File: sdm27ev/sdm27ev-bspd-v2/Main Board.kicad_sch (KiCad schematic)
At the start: 41 parts, among them IC201 74AHC1G08, IC202 SN74LVC1G17DBVRG4, IC203 SN74HC32PWR, IC204 L7805ACD2T-TR, U201 TLV9022QDRQ1

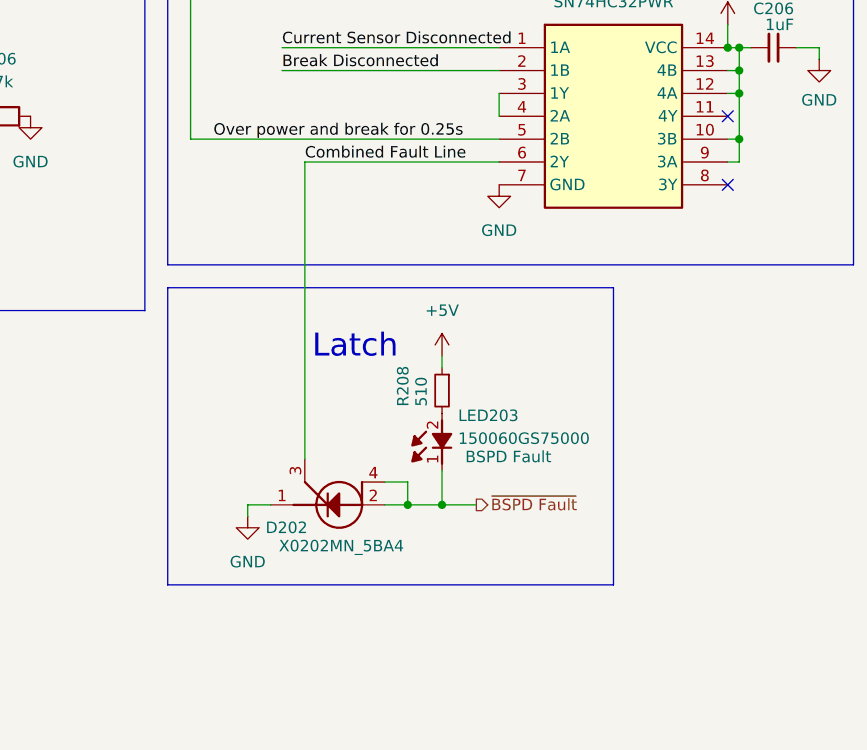
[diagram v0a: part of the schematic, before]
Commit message: Fixed? latch logic voltage levels
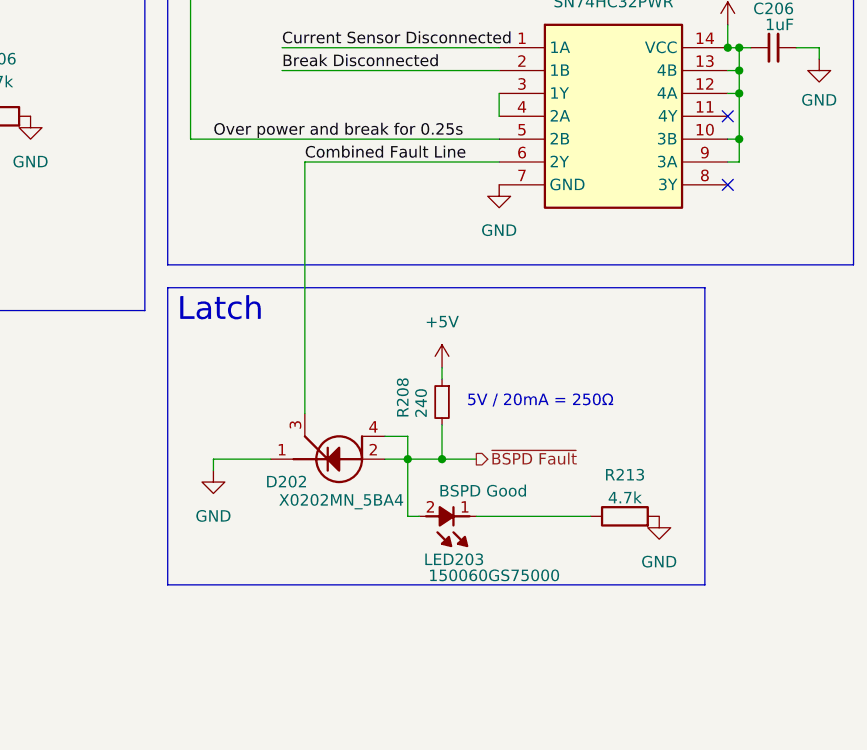
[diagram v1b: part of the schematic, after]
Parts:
- added R213: 4.7k, Resistor_SMD:R_0603_1608Metric, symbol Device:R
- LED203: Measure BSPD Fault -> BSPD Good
- R208: value 510 -> 240
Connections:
- net GND: now also R213.2
- net ~{BSPD Fault}: now also LED203.2 (A), R208.2; no longer LED203.1 (K)
- new net: LED203.1 (K), R213.1
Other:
- note added: "5V / 20mA = 250Ω"
- moved on the sheet: D202, R208
